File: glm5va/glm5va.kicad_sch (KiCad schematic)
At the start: 21 parts, among them J1 BANK_xx1, J2 JIN, J3 POWER, U1 74HC245, U2 74HC245

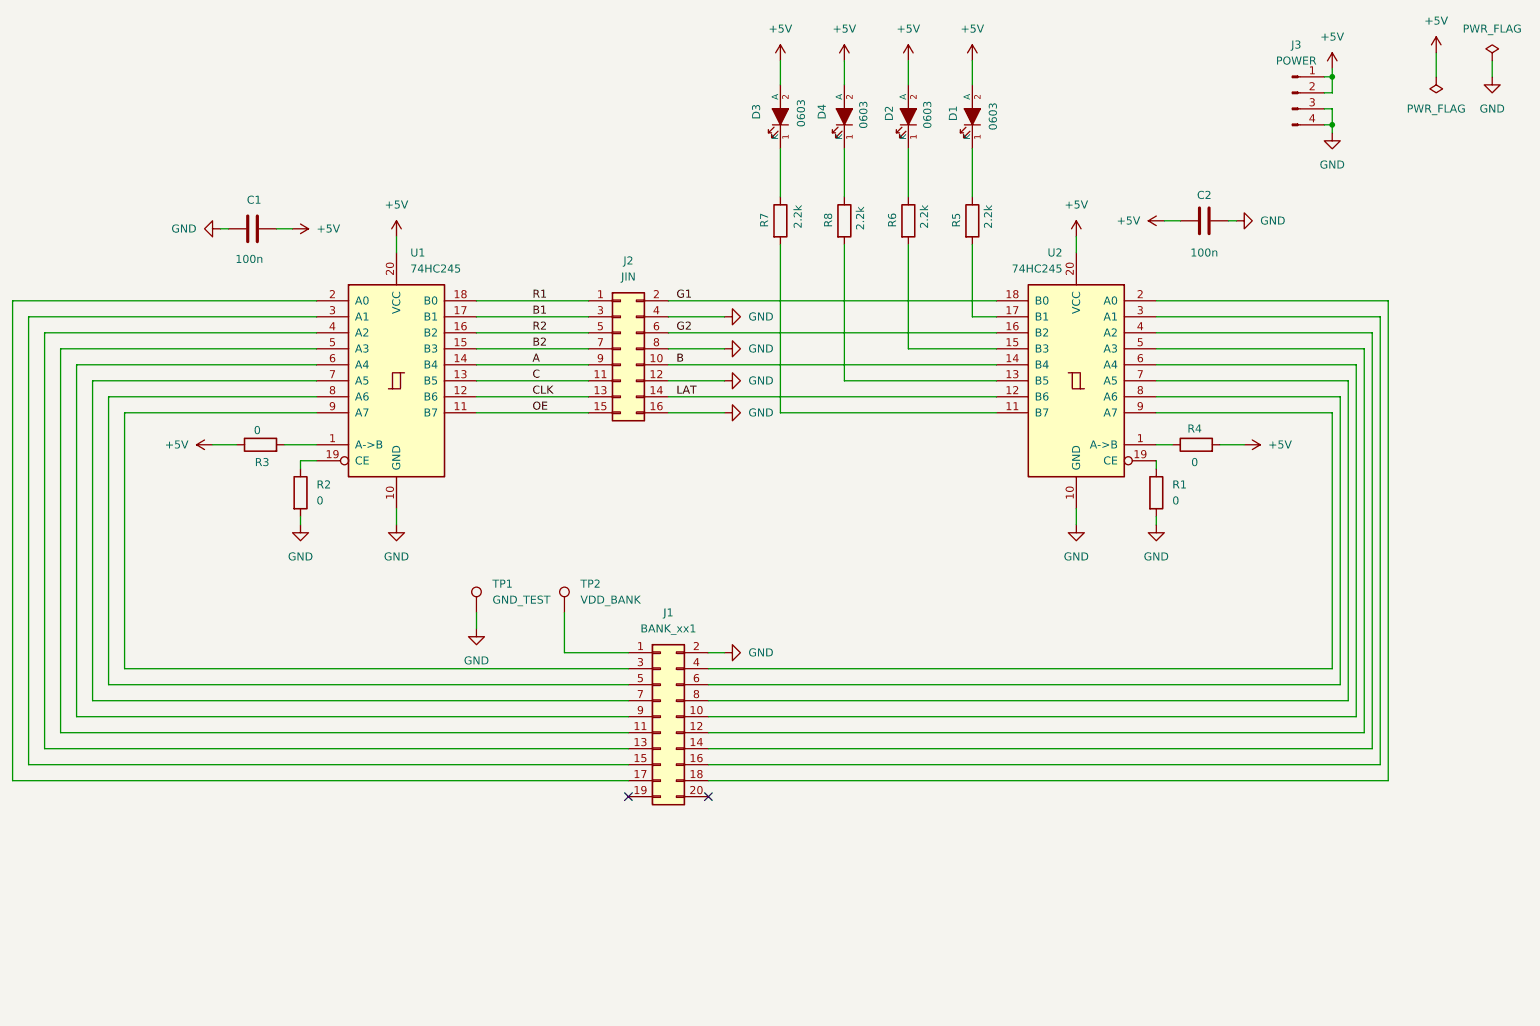
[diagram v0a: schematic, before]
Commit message: glm5va: routing and layers ok
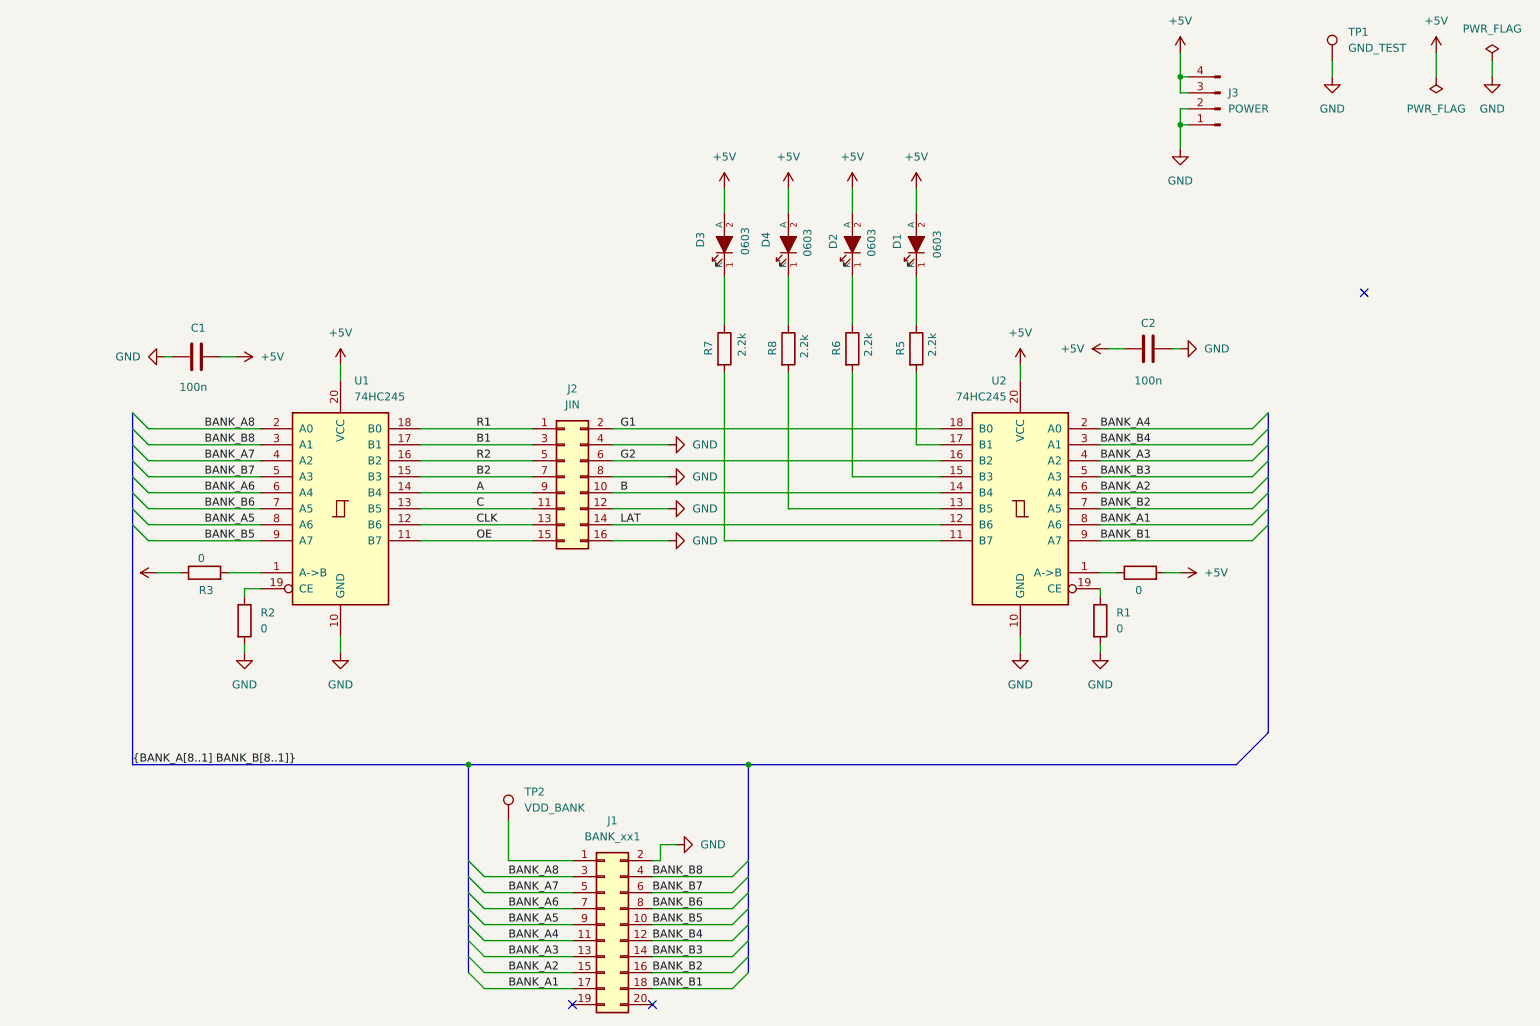
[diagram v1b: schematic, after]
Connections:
- net +5V: now also J3.3 (Pin_3), J3.4 (Pin_4); no longer J3.1 (Pin_1), J3.2 (Pin_2)
- net GND: now also J3.1 (Pin_1), J3.2 (Pin_2); no longer J3.3 (Pin_3), J3.4 (Pin_4)
- net BANK_A1: now reaches J1.17 (Pin_17)
- net BANK_A1: now also U2.8 (A6); no longer U1.2 (A0)
- net BANK_A2: now reaches J1.15 (Pin_15)
- net BANK_A2: now also U2.6 (A4); no longer U1.3 (A1)
- net BANK_A3: now reaches J1.13 (Pin_13)
- net BANK_A3: now also U2.4 (A2); no longer U1.4 (A2)
- net BANK_A4: now reaches J1.11 (Pin_11)
- net BANK_A4: now also U2.2 (A0); no longer U1.5 (A3)
- net BANK_A5: now reaches J1.9 (Pin_9)
- net BANK_A5: now also U1.8 (A6); no longer U1.6 (A4)
- net BANK_A6: now reaches J1.7 (Pin_7)
- net BANK_A6: now also U1.6 (A4); no longer U1.7 (A5)
- net BANK_A7: now reaches J1.5 (Pin_5)
- net BANK_A7: now also U1.4 (A2); no longer U1.8 (A6)
- net BANK_A8: now reaches J1.3 (Pin_3)
- net BANK_A8: now also U1.2 (A0); no longer U1.9 (A7)
- net BANK_B5: now reaches J1.10 (Pin_10)
- net BANK_B5: now also U1.9 (A7); no longer U2.6 (A4)
- net BANK_B3: now reaches U2.5 (A3)
- net BANK_B3: now also J1.14 (Pin_14); no longer J1.12 (Pin_12)
- net BANK_B2: now reaches J1.16 (Pin_16)
- net BANK_B2: now also U2.7 (A5); no longer U2.3 (A1)
- net BANK_B1: now reaches J1.18 (Pin_18)
- net BANK_B1: now also U2.9 (A7); no longer U2.2 (A0)
- net BANK_B8: now reaches J1.4 (Pin_4)
- net BANK_B8: now also U1.3 (A1); no longer U2.9 (A7)
- net BANK_B7: now reaches J1.6 (Pin_6)
- net BANK_B7: now also U1.5 (A3); no longer U2.8 (A6)
- net BANK_B6: now reaches J1.8 (Pin_8)
- net BANK_B6: now also U1.7 (A5); no longer U2.7 (A5)
- new net BANK_B4: J1.12 (Pin_12), U2.3 (A1)
- no-connect marks 2 -> 3
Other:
- moved on the sheet: C1, C2, D1, D2, D3, D4, J1, J2, J3, R1, R2, R3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
